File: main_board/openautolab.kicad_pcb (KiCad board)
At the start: 2 copper layers, 144.8 x 88.9 mm, 35 parts, among them J1 PIN11, J10 HX711, J11 LCD, J16 PWR_IN, J17 FILTER_PUMP, J18 FILTER_SENSOR, J2 PIN9, J3 PIN10, J4 PIN12, J6 PIN7, J7 PIN8, J8 PUMP, J9 SERVO, K1 FINDER-36.11, K2 FINDER-36.11, SW0 PIN_A0, SW1 PIN_A1, SW2 PIN_A2, SW3 SW_DPST_x2, SW4 SW_DPST_x2, U1 TD62064APG, U2 TD62064APG, U3 LM2576T-5

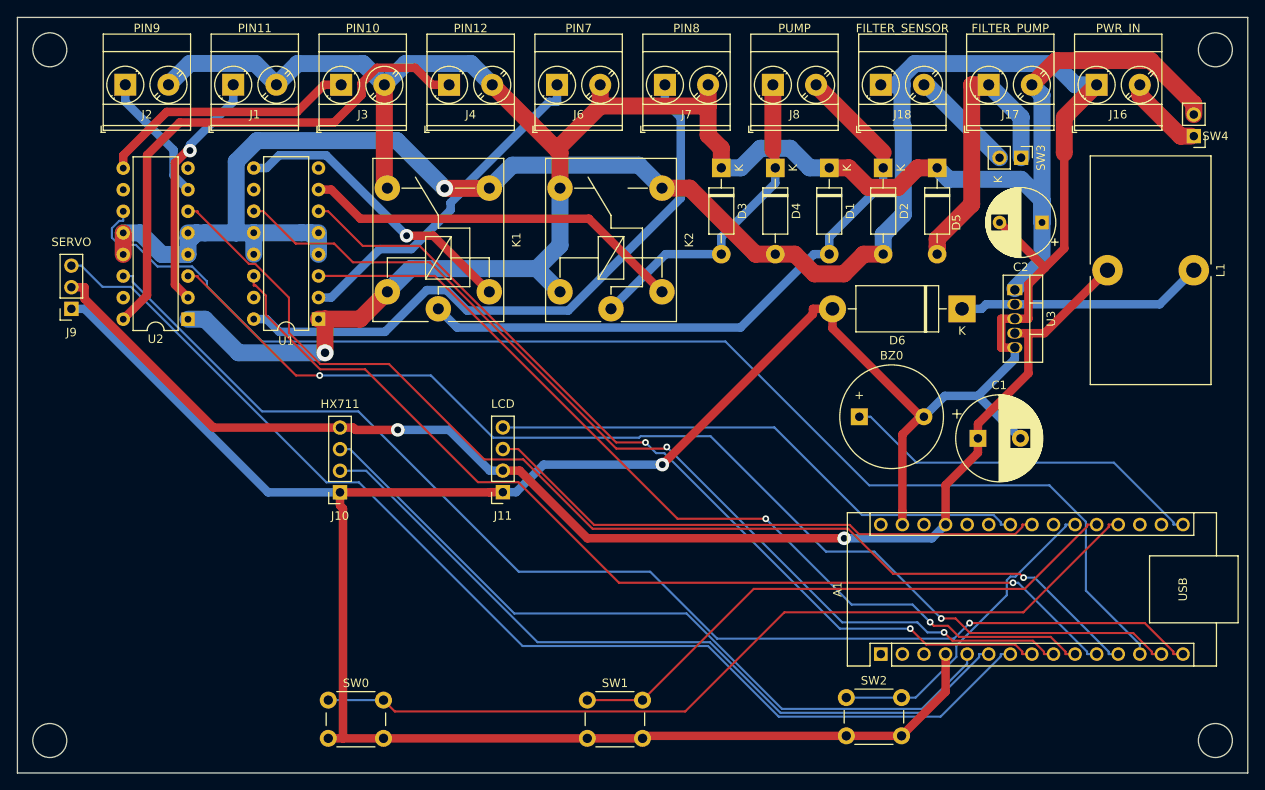
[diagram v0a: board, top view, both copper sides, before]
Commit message: update board
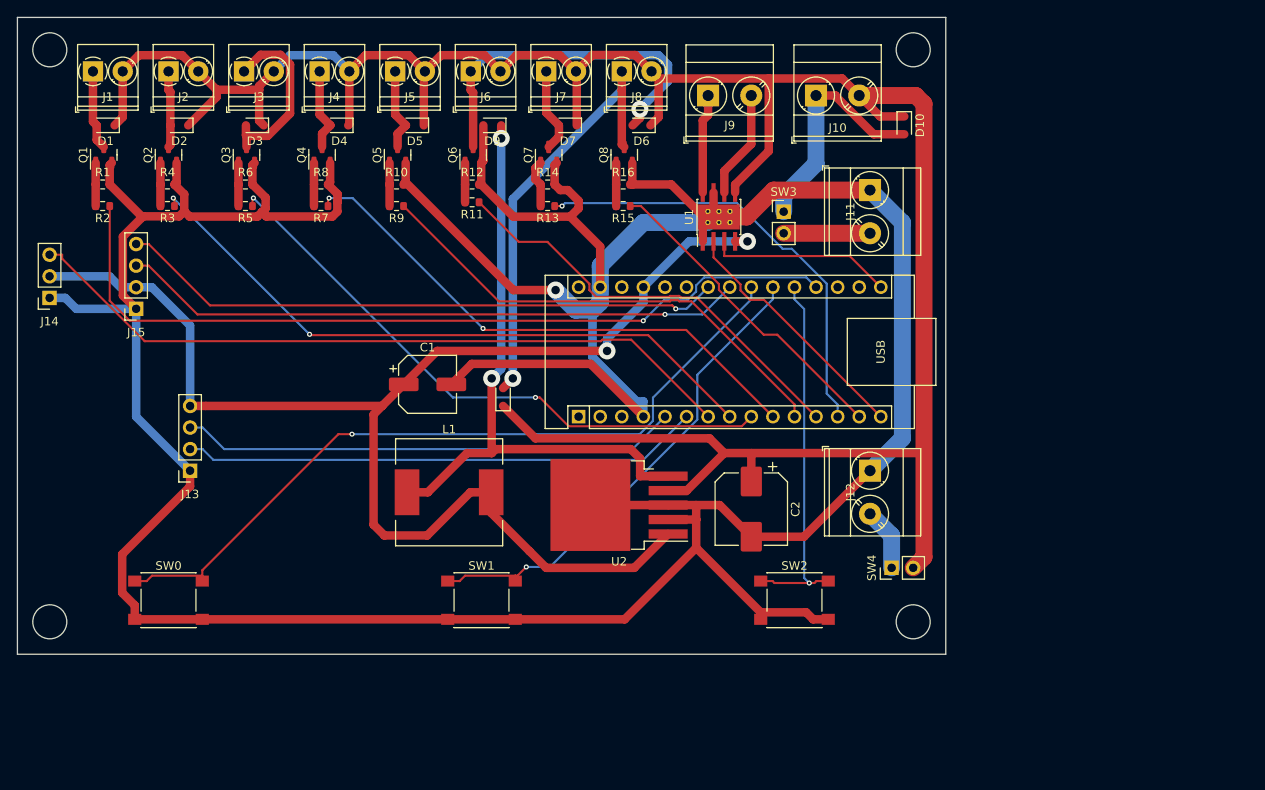
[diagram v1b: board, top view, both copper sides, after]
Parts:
- removed BZ0: Buzzer, Buzzer_Beeper:Buzzer_12x9.5RM7.6
- removed J16: PWR_IN, TerminalBlock_Phoenix:TerminalBlock_Phoenix_MKDS-3-2-5.08_1x02_P5.08mm_Horizontal
- removed J17: FILTER_PUMP, TerminalBlock_Phoenix:TerminalBlock_Phoenix_MKDS-3-2-5.08_1x02_P5.08mm_Horizontal
- removed J18: FILTER_SENSOR, TerminalBlock_Phoenix:TerminalBlock_Phoenix_MKDS-3-2-5.08_1x02_P5.08mm_Horizontal
- removed K1, K2: FINDER-36.11, Relay_THT:Relay_SPDT_Finder_36.11
- removed NT1: NetTie_2, NetTie:NetTie-2_SMD_Pad2.0mm
- removed U3: LM2576T-5, Package_TO_SOT_THT:TO-220-5_Vertical
- added D10: 1N5819WS, Diode_SMD:D_SOD-323, F.Cu at (138.7, 49.5)
- added D7: 1N5819WS, Diode_SMD:D_SOD-323, F.Cu at (99.1, 49.5)
- added D8: 1N5819WS, Diode_SMD:D_SOD-323, F.Cu at (91.4, 81.5)
- added D9: 1N5819, Diode_SMD:D_SOD-323, F.Cu at (90.2, 49.5)
- added J12: PWR_IN, TerminalBlock_Phoenix:TerminalBlock_Phoenix_MKDS-3-2-5.08_1x02_P5.08mm_Horizontal, F.Cu at (134.6, 90.2)
- added J13: HX711, Connector_PinSocket_2.54mm:PinSocket_1x04_P2.54mm_Vertical, F.Cu at (54.6, 90.2)
- added J14: SERVO, Connector_PinSocket_2.54mm:PinSocket_1x03_P2.54mm_Vertical, F.Cu at (38.1, 69.8)
- added J15: LCD, Connector_PinSocket_2.54mm:PinSocket_1x04_P2.54mm_Vertical, F.Cu at (48.3, 71.1)
- added J5: PIN9, TerminalBlock_Phoenix:TerminalBlock_Phoenix_PT-1,5-2-3.5-H_1x02_P3.50mm_Horizontal, F.Cu at (78.7, 43.2)
- added Q1: TSM2302CX, Package_TO_SOT_SMD:SOT-23, F.Cu at (44.5, 53.0)
- added Q2: TSM2302CX, Package_TO_SOT_SMD:SOT-23, F.Cu at (52.1, 53.0)
- added Q3: TSM2302CX, Package_TO_SOT_SMD:SOT-23, F.Cu at (61.2, 53.0)
- added Q4: TSM2302CX, Package_TO_SOT_SMD:SOT-23, F.Cu at (70.1, 53.0)
- added Q5: TSM2302CX, Package_TO_SOT_SMD:SOT-23, F.Cu at (79.0, 53.0)
- added Q6: TSM2302CX, Package_TO_SOT_SMD:SOT-23, F.Cu at (87.9, 53.0)
- added Q7: TSM2302CX, Package_TO_SOT_SMD:SOT-23, F.Cu at (96.8, 53.0)
- added Q8: TSM2302CX, Package_TO_SOT_SMD:SOT-23, F.Cu at (105.7, 53.0)
- added R1: 10k, Resistor_SMD:R_0603_1608Metric, F.Cu at (44.3, 56.5)
- added R10: 10k, Resistor_SMD:R_0603_1608Metric, F.Cu at (78.9, 56.5)
- added R11: 100, Resistor_SMD:R_0603_1608Metric, F.Cu at (87.8, 58.6)
- added R12: 10k, Resistor_SMD:R_0603_1608Metric, F.Cu at (87.8, 56.5)
- added R13: 100, Resistor_SMD:R_0603_1608Metric, F.Cu at (96.7, 59.0)
- added R14: 10k, Resistor_SMD:R_0603_1608Metric, F.Cu at (96.7, 56.5)
- added R15: 100, Resistor_SMD:R_0603_1608Metric, F.Cu at (105.6, 59.0)
- added R16: 10k, Resistor_SMD:R_0603_1608Metric, F.Cu at (105.6, 56.5)
- added R2: 100, Resistor_SMD:R_0603_1608Metric, F.Cu at (44.3, 59.0)
- added R3: 100, Resistor_SMD:R_0603_1608Metric, F.Cu at (51.9, 59.0)
- added R4: 10k, Resistor_SMD:R_0603_1608Metric, F.Cu at (51.9, 56.5)
- added R5: 100, Resistor_SMD:R_0603_1608Metric, F.Cu at (61.1, 59.0)
- added R6: 10k, Resistor_SMD:R_0603_1608Metric, F.Cu at (61.1, 56.5)
- added R7: 100, Resistor_SMD:R_0603_1608Metric, F.Cu at (70.0, 59.0)
- added R8: 10k, Resistor_SMD:R_0603_1608Metric, F.Cu at (70.0, 56.5)
- added R9: 100, Resistor_SMD:R_0603_1608Metric, F.Cu at (78.9, 59.0)
- C1: value C_Polarized -> 100; footprint Capacitor_THT:CP_Radial_D10.0mm_P5.00mm -> Capacitor_SMD:CP_Elec_6.3x5.4
- C2: value C_Polarized -> 330; footprint Capacitor_THT:CP_Radial_D8.0mm_P5.00mm -> Capacitor_SMD:CP_Elec_8x10
- D1, D2, D3, D4, D5: value 1N4004 -> 1N5819WS; footprint Diode_THT:D_DO-41_SOD81_P10.16mm_Horizontal -> Diode_SMD:D_SOD-323
- D6: value 1N5822 -> 1N5819WS; footprint Diode_THT:D_DO-201AD_P15.24mm_Horizontal -> Diode_SMD:D_SOD-323
- J1: value PIN11 -> PIN13; footprint TerminalBlock_Phoenix:TerminalBlock_Phoenix_MKDS-3-2-5.08_1x02_P5.08mm_Horizontal -> TerminalBlock_Phoenix:TerminalBlock_Phoenix_PT-1,5-2-3.5-H_1x02_P3.50mm_Horizontal
- J10: value HX711 -> FILTER_PUMP; footprint Connector_PinSocket_2.54mm:PinSocket_1x04_P2.54mm_Vertical -> TerminalBlock_Phoenix:TerminalBlock_Phoenix_MKDS-3-2-5.08_1x02_P5.08mm_Horizontal
- J11: value LCD -> FILTER_SENSOR; footprint Connector_PinSocket_2.54mm:PinSocket_1x04_P2.54mm_Vertical -> TerminalBlock_Phoenix:TerminalBlock_Phoenix_MKDS-3-2-5.08_1x02_P5.08mm_Horizontal
- J2: value PIN9 -> PIN12; footprint TerminalBlock_Phoenix:TerminalBlock_Phoenix_MKDS-3-2-5.08_1x02_P5.08mm_Horizontal -> TerminalBlock_Phoenix:TerminalBlock_Phoenix_PT-1,5-2-3.5-H_1x02_P3.50mm_Horizontal
- J3: value PIN10 -> PIN11; footprint TerminalBlock_Phoenix:TerminalBlock_Phoenix_MKDS-3-2-5.08_1x02_P5.08mm_Horizontal -> TerminalBlock_Phoenix:TerminalBlock_Phoenix_PT-1,5-2-3.5-H_1x02_P3.50mm_Horizontal
- J4: value PIN12 -> PIN10; footprint TerminalBlock_Phoenix:TerminalBlock_Phoenix_MKDS-3-2-5.08_1x02_P5.08mm_Horizontal -> TerminalBlock_Phoenix:TerminalBlock_Phoenix_PT-1,5-2-3.5-H_1x02_P3.50mm_Horizontal
- J6: value PIN7 -> PIN8; footprint TerminalBlock_Phoenix:TerminalBlock_Phoenix_MKDS-3-2-5.08_1x02_P5.08mm_Horizontal -> TerminalBlock_Phoenix:TerminalBlock_Phoenix_PT-1,5-2-3.5-H_1x02_P3.50mm_Horizontal
- J7: value PIN8 -> PIN7; footprint TerminalBlock_Phoenix:TerminalBlock_Phoenix_MKDS-3-2-5.08_1x02_P5.08mm_Horizontal -> TerminalBlock_Phoenix:TerminalBlock_Phoenix_PT-1,5-2-3.5-H_1x02_P3.50mm_Horizontal
- J8: value PUMP -> PINA0; footprint TerminalBlock_Phoenix:TerminalBlock_Phoenix_MKDS-3-2-5.08_1x02_P5.08mm_Horizontal -> TerminalBlock_Phoenix:TerminalBlock_Phoenix_PT-1,5-2-3.5-H_1x02_P3.50mm_Horizontal
- J9: value SERVO -> PUMP; footprint Connector_PinSocket_2.54mm:PinSocket_1x03_P2.54mm_Vertical -> TerminalBlock_Phoenix:TerminalBlock_Phoenix_MKDS-3-2-5.08_1x02_P5.08mm_Horizontal
- L1: value L -> 330; footprint Inductor_THT:L_Toroid_Vertical_L26.7mm_W14.0mm_P10.16mm_Pulse_D -> Inductor_SMD:L_12x12mm_H8mm
- SW0, SW1, SW2: footprint Button_Switch_THT:SW_PUSH_6mm -> Button_Switch_SMD:SW_Push_1P1T_NO_6x6mm_H9.5mm
- U1: value TD62064APG -> DRV8870DDA; footprint Package_DIP:DIP-16_W7.62mm -> Package_SO:Texas_HTSOP-8-1EP_3.9x4.9mm_P1.27mm_EP2.95x4.9mm_Mask2.4x3.1mm_ThermalVias
- U2: value TD62064APG -> LM2575-5.0BU; footprint Package_DIP:DIP-16_W7.62mm -> Package_TO_SOT_SMD:TO-263-5_TabPin3
- moved L1 91.4 mm to (85.1, 92.7), turned to 0 degrees
- moved D1 85.3 mm to (44.7, 49.5), turned to 180 degrees
- moved D2 83.0 mm to (53.3, 49.5), turned to 180 degrees
- moved J9 79.0 mm to (115.6, 46.0), turned to 0 degrees
- moved J10 72.9 mm to (128.3, 46.0), turned to 0 degrees
- moved C1 65.1 mm to (82.5, 80.0)
- moved SW4 62.0 mm to (137.2, 101.6), turned to 90 degrees
- moved D5 61.7 mm to (81.1, 49.5), turned to 180 degrees
- moved J11 56.0 mm to (134.6, 57.1), turned to -90 degrees
- moved U2 55.2 mm to (105.1, 94.2)
- moved D3 55.1 mm to (62.2, 49.5), turned to 180 degrees
- moved D4 51.5 mm to (72.2, 49.5), turned to 180 degrees
- moved U1 48.6 mm to (116.8, 60.3), turned to 90 degrees
- moved C2 48.0 mm to (120.7, 94.7), turned to -90 degrees
- moved A1 45.2 mm to (100.3, 83.8)
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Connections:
- A1 pad 22: unconnected-(A1-A3-Pad22) -> Net-(A1-A3)
- D2 pad 1: Net-(D1-A) -> +12V
- D2 pad 2: GNDPWR -> Net-(D2-A)
- D4 pad 1: Net-(D3-A) -> +12V
- D4 pad 2: GNDPWR -> Net-(D4-A)
- D6 pad 1: Net-(D6-K) -> +12V
- D6 pad 2: GND -> Net-(D6-A)
- J1 pad 1: Net-(J1-Pin_1) -> Net-(D1-A)
- J10 pad 1: GND -> Net-(D10-A)
- J10 pad 2: Net-(A1-D3) -> +12V
- J11 pad 2: +5V -> Net-(J11-Pin_2)
- J2 pad 1: Net-(J2-Pin_1) -> Net-(D2-A)
- J3 pad 1: Net-(J3-Pin_1) -> Net-(D3-A)
- J4 pad 1: Net-(J4-Pin_1) -> Net-(D4-A)
- J6 pad 1: Net-(J6-Pin_1) -> Net-(D6-A)
- J7 pad 1: Net-(J7-Pin_1) -> Net-(D7-A)
- J8 pad 1: Net-(D3-A) -> Net-(D8-A)
- J8 pad 2: Net-(D1-A) -> +12V
- J9 pad 1: GND -> Net-(J9-Pin_1)
- J9 pad 2: +5V -> Net-(J9-Pin_2)
- L1 pad 1: Net-(D6-K) -> Net-(D9-K)
- SW0 pad 1: Net-(A1-A0) -> Net-(A1-A3)
- SW1 pad 1: Net-(A1-A1) -> Net-(A1-A2)
- SW2 pad 1: Net-(A1-A2) -> Net-(A1-A1)
- SW3 pad 1: Net-(D5-A) -> Net-(D10-A)
- SW3 pad 2: Net-(J18-Pin_2) -> Net-(J11-Pin_2)
- U1 pad 1: +12V -> GND
- U1 pad 2: Net-(J6-Pin_1) -> Net-(A1-D12)
- U1 pad 3: Net-(A1-D7) -> Net-(A1-D13)
- U1 pad 4: GNDPWR -> +5V
- U1 pad 5: GNDPWR -> +12V
- U1 pad 6: Net-(A1-D5) -> Net-(J9-Pin_2)
- U1 pad 7: Net-(U1-O2) -> GND
- U1 pad 8: (no net) -> Net-(J9-Pin_1)
- U1 pad 9: Net-(U1-O3) -> GND
- U2 pad 1: +12V -> +5V
- U2 pad 2: Net-(J1-Pin_1) -> GND
- U2 pad 3: Net-(A1-D11) -> GND
- U2 pad 4: GNDPWR -> +12V
- U2 pad 5: GNDPWR -> Net-(D9-K)
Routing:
- net GNDPWR: track 185.2 -> 0.00 mm, vias 1 -> 0
- net GND: track 306.1 -> 466.2 mm
- net Net-(A1-D12): track 145.2 -> 29.7 mm, vias 1 -> 0
- net Net-(A1-D10): track 150.9 -> 52.3 mm, vias 0 -> 1
- net Net-(A1-D11): track 133.4 -> 37.6 mm, vias 2 -> 0
- net Net-(A1-A3): track 0.00 -> 90.3 mm, vias 0 -> 1
- net Net-(A1-D9): track 133.7 -> 50.6 mm, vias 1 -> 0
- net Net-(D9-K): track 0.00 -> 74.4 mm, vias 0 -> 2
- net Net-(J7-Pin_1): track 73.5 -> 0.00 mm
- net Net-(D1-A): track 76.3 -> 9.42 mm
- net Net-(A1-D8): track 119.8 -> 57.2 mm, vias 1 -> 0
- net Net-(J4-Pin_1): track 61.9 -> 0.00 mm
- net Net-(D8-A): track 0.00 -> 52.1 mm, vias 0 -> 1
- net Net-(A1-D4): track 135.7 -> 85.8 mm
- net Net-(U1-O2): track 45.4 -> 0.00 mm
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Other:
- board size 144.8 x 88.9 mm -> 109.2 x 74.9 mm
